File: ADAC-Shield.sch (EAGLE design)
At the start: 58 parts, among them U1 ARDUINO-MEGAFULL, U2 LM358D

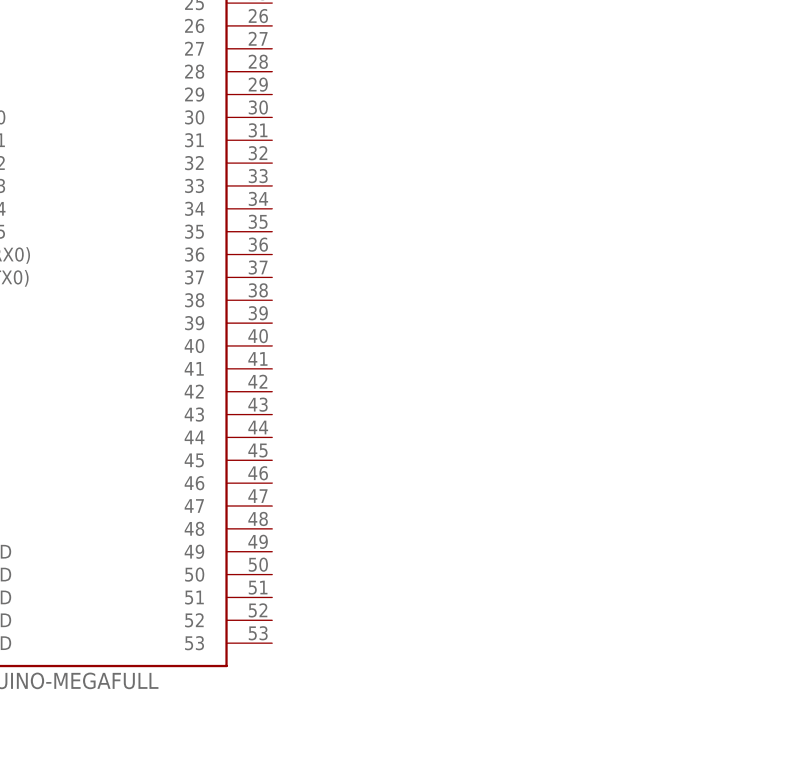
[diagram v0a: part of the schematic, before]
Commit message: Board layout finished for v0.1
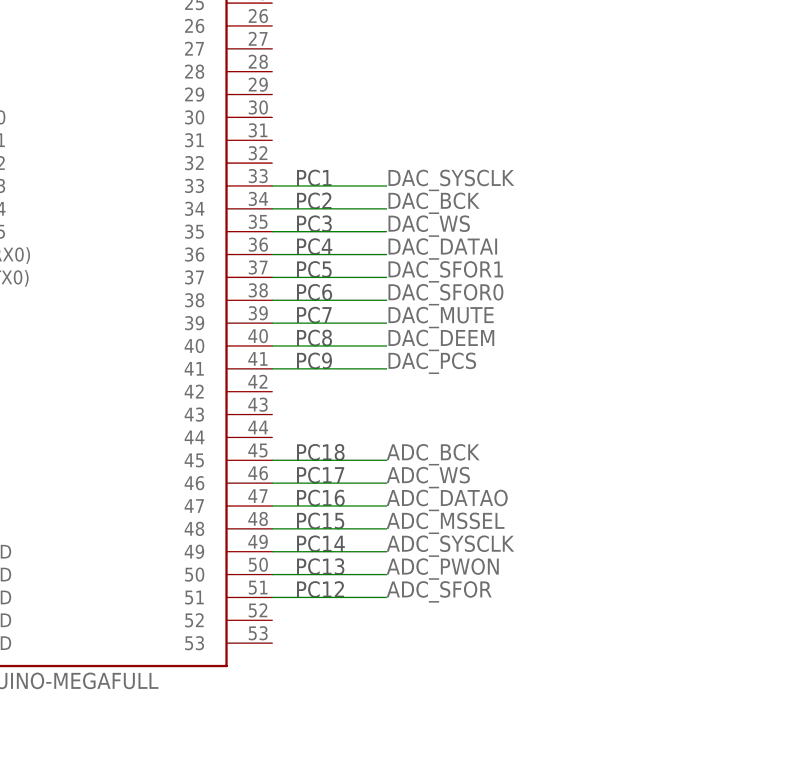
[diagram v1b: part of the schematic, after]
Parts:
- U1: device SparkFun-Boards:ARDUINO-MEGAFULL -> SparkFun-Boards_modified:ARDUINO-MEGAFULL
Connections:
- net ADC_BCK: now also U1.45
- net ADC_DATAO: now also U1.47
- net ADC_MSSEL: now also U1.48
- net ADC_PWON: now also U1.50
- net ADC_SFOR: now also U1.51
- net ADC_SYSCLK: now also U1.49
- net ADC_WS: now also U1.46
- net DAC_BCK: now also U1.34
- net DAC_DATAI: now also U1.36
- net DAC_DEEM: now also U1.40
- net DAC_MUTE: now also U1.39
- net DAC_PCS: now also U1.41
- net DAC_SFOR0: now also U1.38
- net DAC_SFOR1: now also U1.37
- net DAC_SYSCLK: now also U1.33
- net DAC_WS: now also U1.35
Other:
- note added: "PC1"
- note added: "PC12"
- note added: "PC13"
- note added: "PC14"
- note added: "PC15"
- note added: "PC16"
- note added: "PC17"
- note added: "PC18"
- note added: "PC2"
- note added: "PC3"
- note added: "PC4"
- note added: "PC5"
- note added: "PC6"
- note added: "PC7"
- note added: "PC8"
- note added: "PC9"
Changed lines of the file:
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@@
 </classes>
 <parts>
-<part name="U1" library="SparkFun-Boards" deviceset="ARDUINO-MEGA" device="FULL"/>
 <part name="U2" library="CircuitHub" deviceset="1680-LM358DT" device="" value="LM358D"/>
 <part name="GND1" library="supply1" deviceset="GND" device=""/>
@@
 <part name="GND31" library="supply1" deviceset="GND" device=""/>
 <part name="JP4" library="pinhead" deviceset="PINHD-1X2" device=""/>
+<part name="U1" library="SparkFun-Boards_modified" deviceset="ARDUINO-MEGA" device="FULL"/>
 </parts>
 <sheets>
@@
 <text x="-63.5" y="53.34" size="1.778" layer="91">Low Gain</text>
 <text x="-66.04" y="-2.54" size="1.778" layer="91">Low Gain</text>
+<text x="-198.12" y="0" size="1.778" layer="97">PC1</text>
+<text x="-198.12" y="-2.54" size="1.778" layer="97">PC2</text>
+<text x="-198.12" y="-5.08" size="1.778" layer="97">PC3</text>
+<text x="-198.12" y="-7.62" size="1.778" layer="97">PC4</text>
+<text x="-198.12" y="-10.16" size="1.778" layer="97">PC5</text>
+<text x="-198.12" y="-12.7" size="1.778" layer="97">PC6</text>
+<text x="-198.12" y="-15.24" size="1.778" layer="97">PC7</text>
+<text x="-198.12" y="-17.78" size="1.778" layer="97">PC8</text>
+<text x="-198.12" y="-20.32" size="1.778" layer="97">PC9</text>
+<text x="-198.12" y="-45.72" size="1.778" layer="97">PC12</text>
+<text x="-198.12" y="-43.18" size="1.778" layer="97">PC13</text>
+<text x="-198.12" y="-40.64" size="1.778" layer="97">PC14</text>
+<text x="-198.12" y="-38.1" size="1.778" layer="97">PC15</text>
+<text x="-198.12" y="-35.56" size="1.778" layer="97">PC16</text>
+<text x="-198.12" y="-33.02" size="1.778" layer="97">PC17</text>
+<text x="-198.12" y="-30.48" size="1.778" layer="97">PC18</text>
 </plain>
 <instances>
-<instance part="U1" gate="G$1" x="-220.98" y="0"/>
 <instance part="U2" gate="-A" x="-99.06" y="55.88"/>
 <instance part="U2" gate="-B" x="-99.06" y="0"/>
@@
 <instance part="GND31" gate="1" x="-106.68" y="-160.02"/>
 <instance part="JP4" gate="G$1" x="-170.18" y="60.96" rot="R270"/>
+<instance part="U1" gate="G$1" x="-220.98" y="0"/>
 </instances>
 <busses>
@@
 <net name="+3V3" class="0">
 <segment>
-<pinref part="U1" gate="G$1" pin="3.3V"/>
 <pinref part="+3V2" gate="G$1" pin="+3V3"/>
 <wire x1="-241.3" y1="40.64" x2="-251.46" y2="40.64" width="0.1524" layer="91"/>
 <wire x1="-251.46" y1="40.64" x2="-251.46" y2="43.18" width="0.1524" layer="91"/>
+<pinref part="U1" gate="G$1" pin="3.3V"/>
 </segment>
 <segment>
@@
 <pinref part="GND2" gate="1" pin="GND"/>
 <wire x1="-248.92" y1="-53.34" x2="-248.92" y2="-50.8" width="0.1524" layer="91"/>
-<pinref part="U1" gate="G$1" pin="GND@0"/>
 <wire x1="-248.92" y1="-50.8" x2="-248.92" y2="-48.26" width="0.1524" layer="91"/>
 <wire x1="-248.92" y1="-48.26" x2="-248.92" y2="-45.72" width="0.1524" layer="91"/>
@@
 <wire x1="-248.92" y1="-43.18" x2="-248.92" y2="-40.64" width="0.1524" layer="91"/>
 <wire x1="-248.92" y1="-40.64" x2="-241.3" y2="-40.64" width="0.1524" layer="91"/>
-<pinref part="U1" gate="G$1" pin="GND@1"/>
 <wire x1="-241.3" y1="-43.18" x2="-248.92" y2="-43.18" width="0.1524" layer="91"/>
 <junction x="-248.92" y="-43.18"/>
-<pinref part="U1" gate="G$1" pin="GND@2"/>
 <wire x1="-241.3" y1="-45.72" x2="-248.92" y2="-45.72" width="0.1524" layer="91"/>
 <junction x="-248.92" y="-45.72"/>
-<pinref part="U1" gate="G$1" pin="GND@3"/>
 <wire x1="-241.3" y1="-48.26" x2="-248.92" y2="-48.26" width="0.1524" layer="91"/>
 <junction x="-248.92" y="-48.26"/>
-<pinref part="U1" gate="G$1" pin="GND@4"/>
 <wire x1="-241.3" y1="-50.8" x2="-248.92" y2="-50.8" width="0.1524" layer="91"/>
 <junction x="-248.92" y="-50.8"/>
+<pinref part="U1" gate="G$1" pin="GND@4"/>
+<pinref part="U1" gate="G$1" pin="GND@0"/>
+<pinref part="U1" gate="G$1" pin="GND@1"/>
+<pinref part="U1" gate="G$1" pin="GND@2"/>
+<pinref part="U1" gate="G$1" pin="GND@3"/>
 </segment>
 <segment>
@@
 <pinref part="S1" gate="S" pin="3"/>
 <wire x1="-256.54" y1="33.02" x2="-256.54" y2="35.56" width="0.1524" layer="91"/>
-<pinref part="U1" gate="G$1" pin="RESET"/>
 <wire x1="-256.54" y1="35.56" x2="-241.3" y2="35.56" width="0.1524" layer="91"/>
 <junction x="-256.54" y="35.56"/>
+<pinref part="U1" gate="G$1" pin="RESET"/>
 </segment>
 </net>
@@
 <label x="-233.68" y="-149.86" size="1.778" layer="95"/>
 </segment>
+<segment>
+<wire x1="-200.66" y1="0" x2="-187.96" y2="0" width="0.1524" layer="91"/>
+<label x="-187.96" y="0" size="1.778" layer="95"/>
+<pinref part="U1" gate="G$1" pin="33"/>
+</segment>
 </net>
 <net name="N$13" class="0">
@@
 <label x="-233.68" y="-154.94" size="1.778" layer="95"/>
 </segment>
+<segment>
+<wire x1="-200.66" y1="-2.54" x2="-187.96" y2="-2.54" width="0.1524" layer="91"/>
+<label x="-187.96" y="-2.54" size="1.778" layer="95"/>
+<pinref part="U1" gate="G$1" pin="34"/>
+</segment>
 </net>
 <net name="DAC_WS" class="0">
@@
 <label x="-233.68" y="-160.02" size="1.778" layer="95"/>
 </segment>
+<segment>
+<wire x1="-200.66" y1="-5.08" x2="-187.96" y2="-5.08" width="0.1524" layer="91"/>
+<label x="-187.96" y="-5.08" size="1.778" layer="95"/>
+<pinref part="U1" gate="G$1" pin="35"/>
+</segment>
 </net>
 <net name="DAC_DATAI" class="0">
@@
 <label x="-233.68" y="-165.1" size="1.778" layer="95"/>
 </segment>
+<segment>
+<wire x1="-200.66" y1="-7.62" x2="-187.96" y2="-7.62" width="0.1524" layer="91"/>
+<label x="-187.96" y="-7.62" size="1.778" layer="95"/>
+<pinref part="U1" gate="G$1" pin="36"/>
+</segment>
 </net>
 <net name="DAC_SFOR1" class="0">
@@
 <label x="-233.68" y="-170.18" size="1.778" layer="95"/>
 </segment>
+<segment>
+<wire x1="-200.66" y1="-10.16" x2="-187.96" y2="-10.16" width="0.1524" layer="91"/>
+<label x="-187.96" y="-10.16" size="1.778" layer="95"/>
+<pinref part="U1" gate="G$1" pin="37"/>
+</segment>
 </net>
 <net name="DAC_SFOR0" class="0">
@@
 <label x="-233.68" y="-175.26" size="1.778" layer="95"/>
 </segment>
+<segment>
+<wire x1="-200.66" y1="-12.7" x2="-187.96" y2="-12.7" width="0.1524" layer="91"/>
+<label x="-187.96" y="-12.7" size="1.778" layer="95"/>
+<pinref part="U1" gate="G$1" pin="38"/>
+</segment>
 </net>
 <net name="DAC_MUTE" class="0">
@@
 <label x="-233.68" y="-180.34" size="1.778" layer="95"/>
 </segment>
+<segment>
+<wire x1="-200.66" y1="-15.24" x2="-187.96" y2="-15.24" width="0.1524" layer="91"/>
+<label x="-187.96" y="-15.24" size="1.778" layer="95"/>
+<pinref part="U1" gate="G$1" pin="39"/>
+</segment>
 </net>
 <net name="DAC_DEEM" class="0">
@@
 <label x="-233.68" y="-185.42" size="1.778" layer="95"/>
 </segment>
+<segment>
+<wire x1="-200.66" y1="-17.78" x2="-187.96" y2="-17.78" width="0.1524" layer="91"/>
+<label x="-187.96" y="-17.78" size="1.778" layer="95"/>
+<pinref part="U1" gate="G$1" pin="40"/>
+</segment>
 </net>
 <net name="DAC_PCS" class="0">
@@
 <wire x1="-200.66" y1="-190.5" x2="-215.9" y2="-190.5" width="0.1524" layer="91"/>
 <label x="-233.68" y="-190.5" size="1.778" layer="95"/>
+</segment>
+<segment>
+<wire x1="-200.66" y1="-20.32" x2="-187.96" y2="-20.32" width="0.1524" layer="91"/>
+<label x="-187.96" y="-20.32" size="1.778" layer="95"/>
+<pinref part="U1" gate="G$1" pin="41"/>
 </segment>
 </net>
@@
 <label x="-15.24" y="-172.72" size="1.778" layer="95"/>
 </segment>
+<segment>
+<wire x1="-200.66" y1="-45.72" x2="-187.96" y2="-45.72" width="0.1524" layer="91"/>
+<label x="-187.96" y="-45.72" size="1.778" layer="95"/>
+<pinref part="U1" gate="G$1" pin="51"/>
+</segment>
 </net>
 <net name="ADC_PWON" class="0">
@@
 <label x="-15.24" y="-177.8" size="1.778" layer="95"/>
 </segment>
+<segment>
+<wire x1="-200.66" y1="-43.18" x2="-187.96" y2="-43.18" width="0.1524" layer="91"/>
+<label x="-187.96" y="-43.18" size="1.778" layer="95"/>
+<pinref part="U1" gate="G$1" pin="50"/>
+</segment>
 </net>
 <net name="ADC_SYSCLK" class="0">
@@
 <wire x1="2.54" y1="-182.88" x2="0" y2="-182.88" width="0.1524" layer="91"/>
 <label x="-15.24" y="-182.88" size="1.778" layer="95"/>
+</segment>
+<segment>
+<wire x1="-200.66" y1="-40.64" x2="-187.96" y2="-40.64" width="0.1524" layer="91"/>
+<label x="-187.96" y="-40.64" size="1.778" layer="95"/>
+<pinref part="U1" gate="G$1" pin="49"/>
 </segment>
 </net>
@@
 <label x="38.1" y="-157.48" size="1.778" layer="95"/>
 </segment>
+<segment>
+<wire x1="-200.66" y1="-38.1" x2="-187.96" y2="-38.1" width="0.1524" layer="91"/>
+<label x="-187.96" y="-38.1" size="1.778" layer="95"/>
+<pinref part="U1" gate="G$1" pin="48"/>
+</segment>
 </net>
 <net name="ADC_DATAO" class="0">
@@
 <label x="38.1" y="-162.56" size="1.778" layer="95"/>
 </segment>
+<segment>
+<wire x1="-200.66" y1="-35.56" x2="-187.96" y2="-35.56" width="0.1524" layer="91"/>
+<label x="-187.96" y="-35.56" size="1.778" layer="95"/>
+<pinref part="U1" gate="G$1" pin="47"/>
+</segment>
 </net>
 <net name="ADC_WS" class="0">
@@
 <label x="38.1" y="-167.64" size="1.778" layer="95"/>
 </segment>
+<segment>
+<wire x1="-200.66" y1="-33.02" x2="-187.96" y2="-33.02" width="0.1524" layer="91"/>
+<label x="-187.96" y="-33.02" size="1.778" layer="95"/>
+<pinref part="U1" gate="G$1" pin="46"/>
+</segment>
 </net>
 <net name="ADC_BCK" class="0">
@@
 <wire x1="35.56" y1="-172.72" x2="38.1" y2="-172.72" width="0.1524" layer="91"/>
 <label x="38.1" y="-172.72" size="1.778" layer="95"/>
+</segment>
+<segment>
+<wire x1="-200.66" y1="-30.48" x2="-187.96" y2="-30.48" width="0.1524" layer="91"/>
+<label x="-187.96" y="-30.48" size="1.778" layer="95"/>
+<pinref part="U1" gate="G$1" pin="45"/>
 </segment>
 </net>
@@
 </sheet>
 </sheets>
+<errors>
+</errors>
 </schematic>
 </drawing>
